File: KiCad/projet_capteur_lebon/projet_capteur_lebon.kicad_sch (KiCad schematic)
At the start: 6 parts, among them J1 Power, J2 Digital/PWM, J3 Analog, J4 Digital/PWM

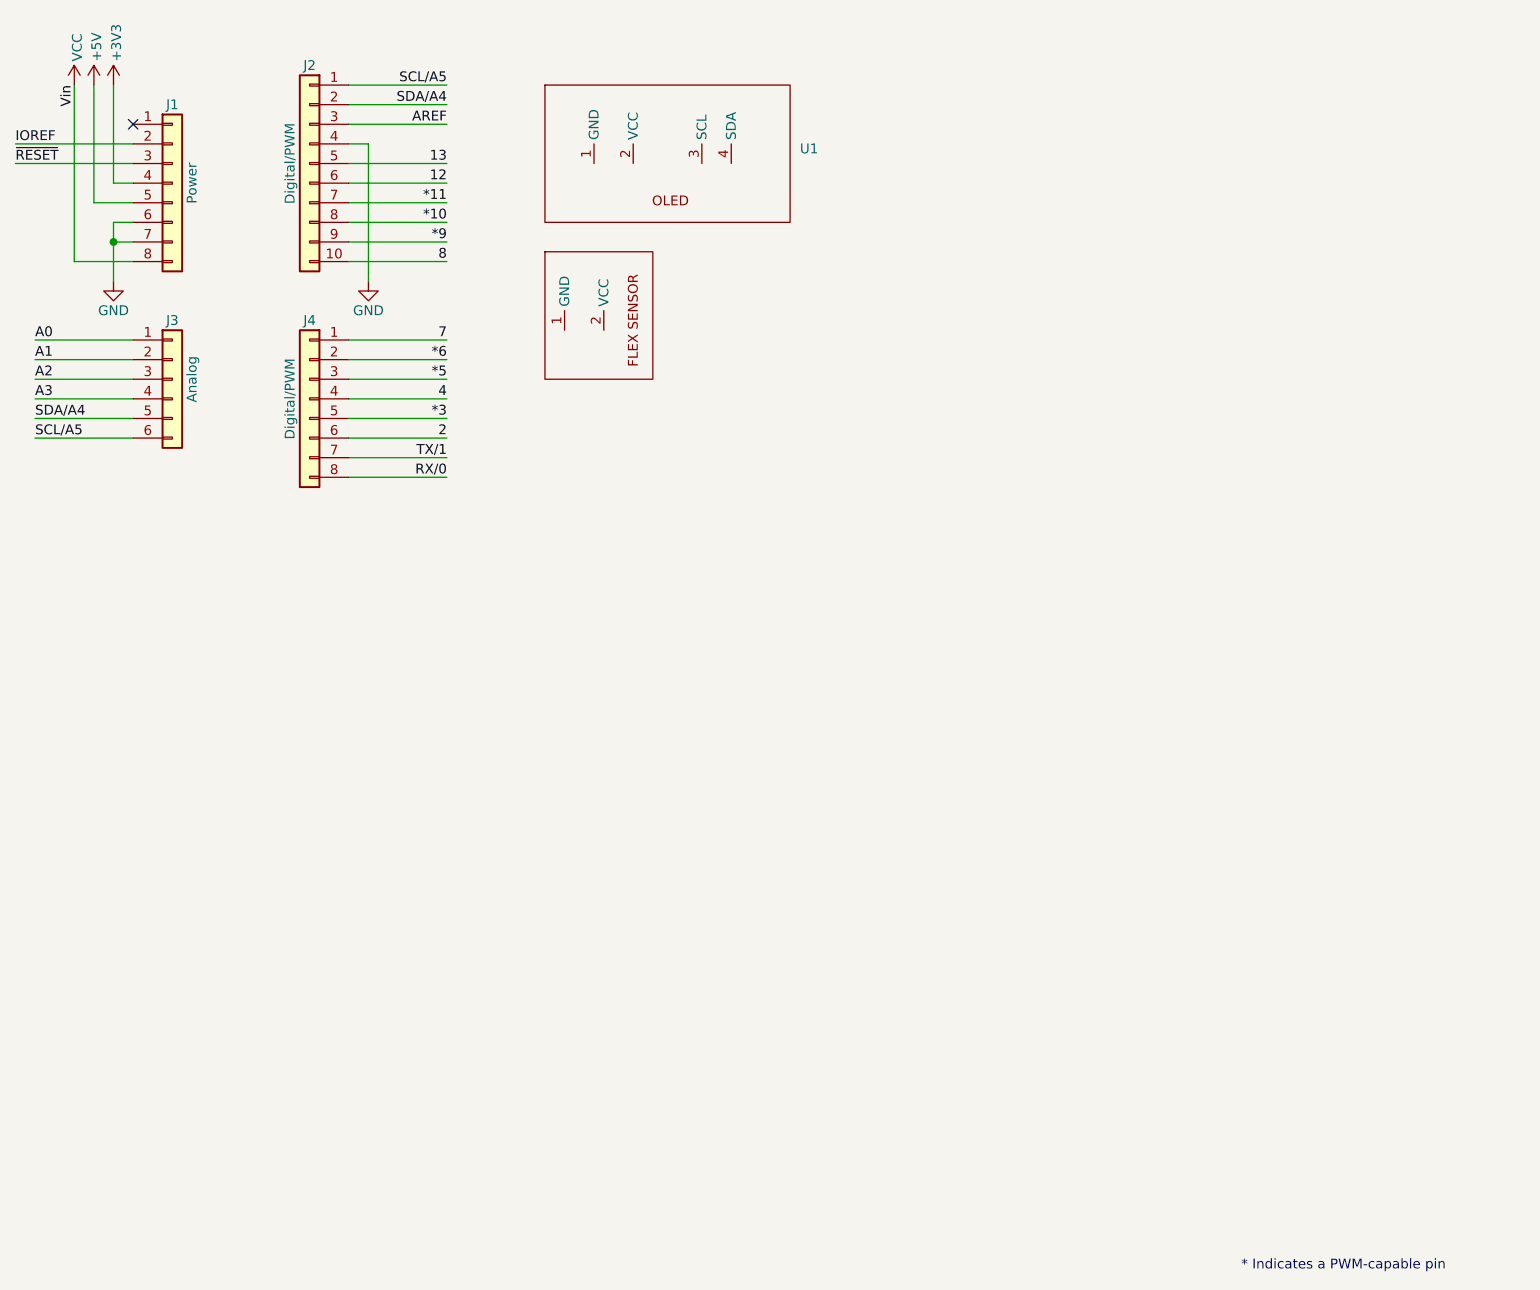
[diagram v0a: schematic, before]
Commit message: creation ampli
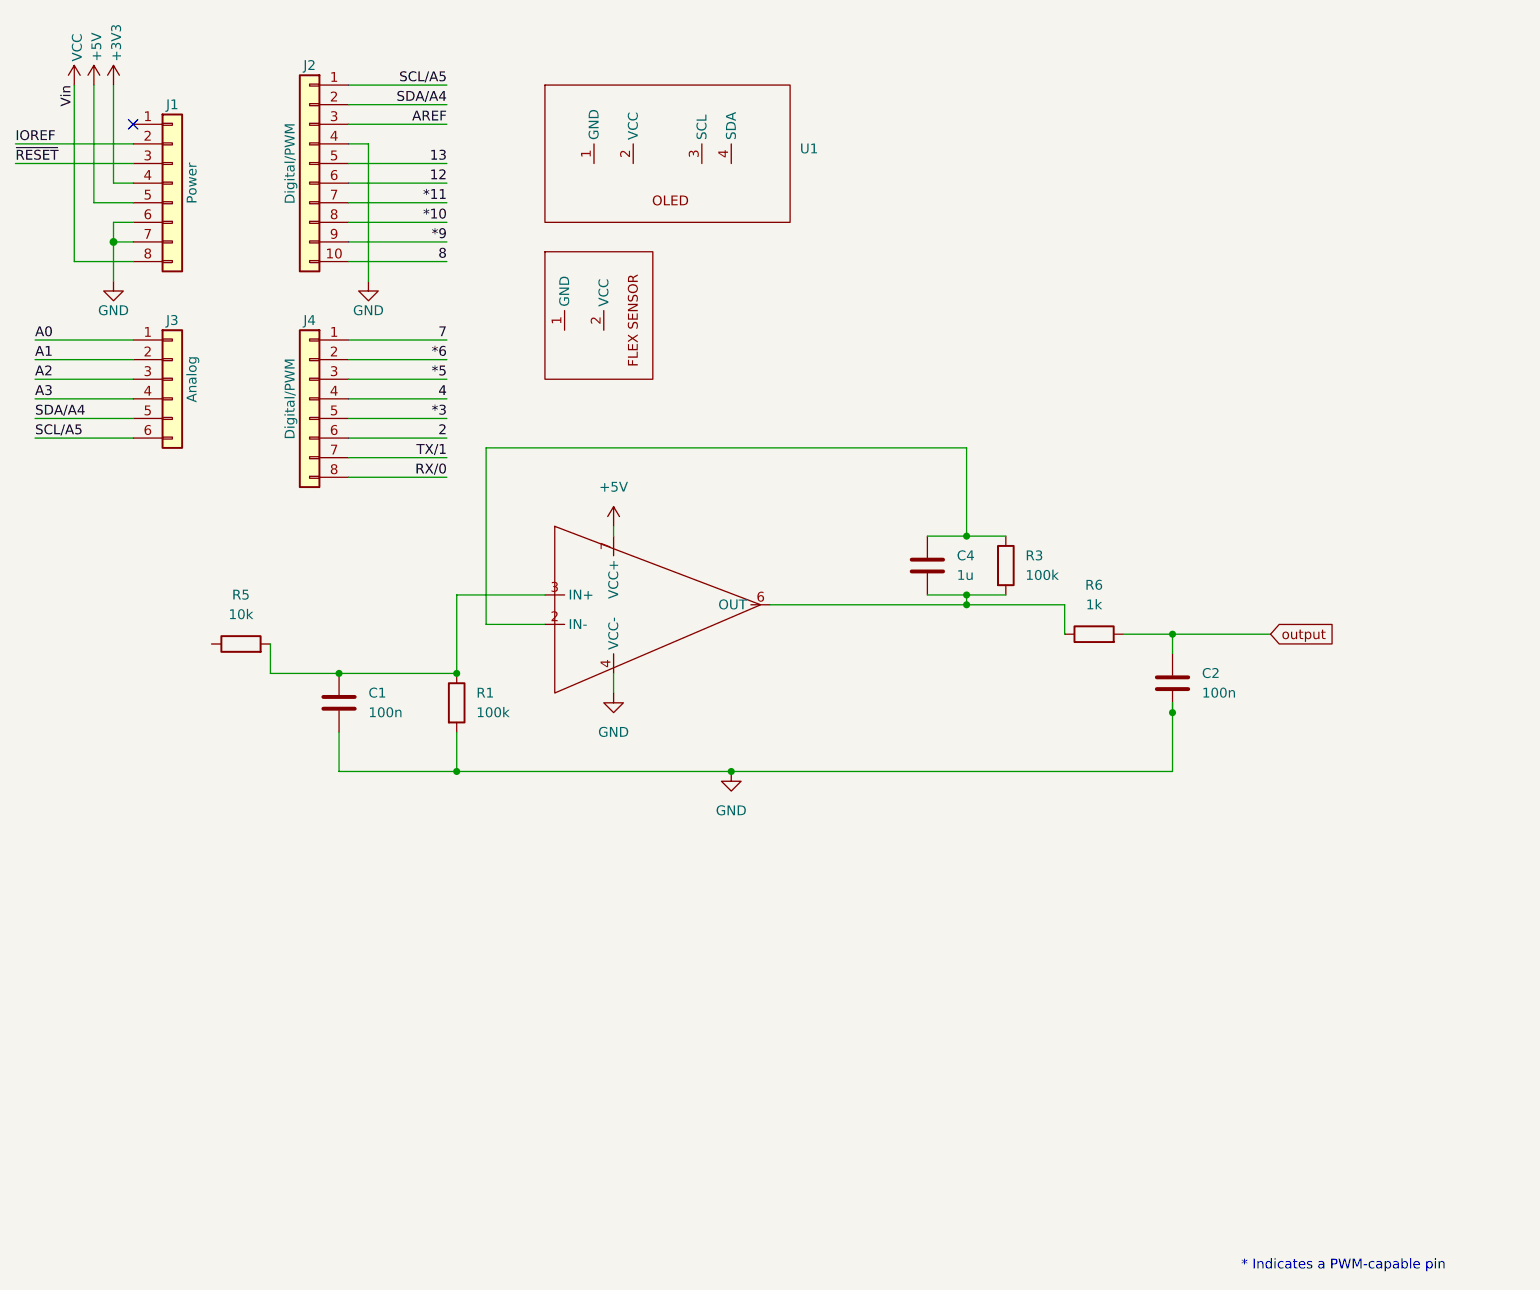
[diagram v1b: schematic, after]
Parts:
- added C1, C2: 100n, symbol Device:C
- added C4: 1u, symbol Device:C
- added R1, R3: 100k, symbol Device:R
- added R5: 10k, symbol Device:R
- added R6: 1k, symbol Device:R
- added U4: ~, librairie_empreintes:DIP-8_296, symbol librairie symboles:AO_LTC1050
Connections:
- net +5V: now also U4.7 (VCC+)
- net GND: now also C1.2, C2.2, R1.2, U4.4 (VCC-)
- new net: C1.1, R1.1, R5.2, U4.3 (IN+)
- new net: C4.1, R3.1, U4.2 (IN-)
- new net: C4.2, R3.2, R6.1, U4.6 (OUT)
- new net output: C2.1, R6.2
